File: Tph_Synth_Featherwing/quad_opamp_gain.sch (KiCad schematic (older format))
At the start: 13 parts

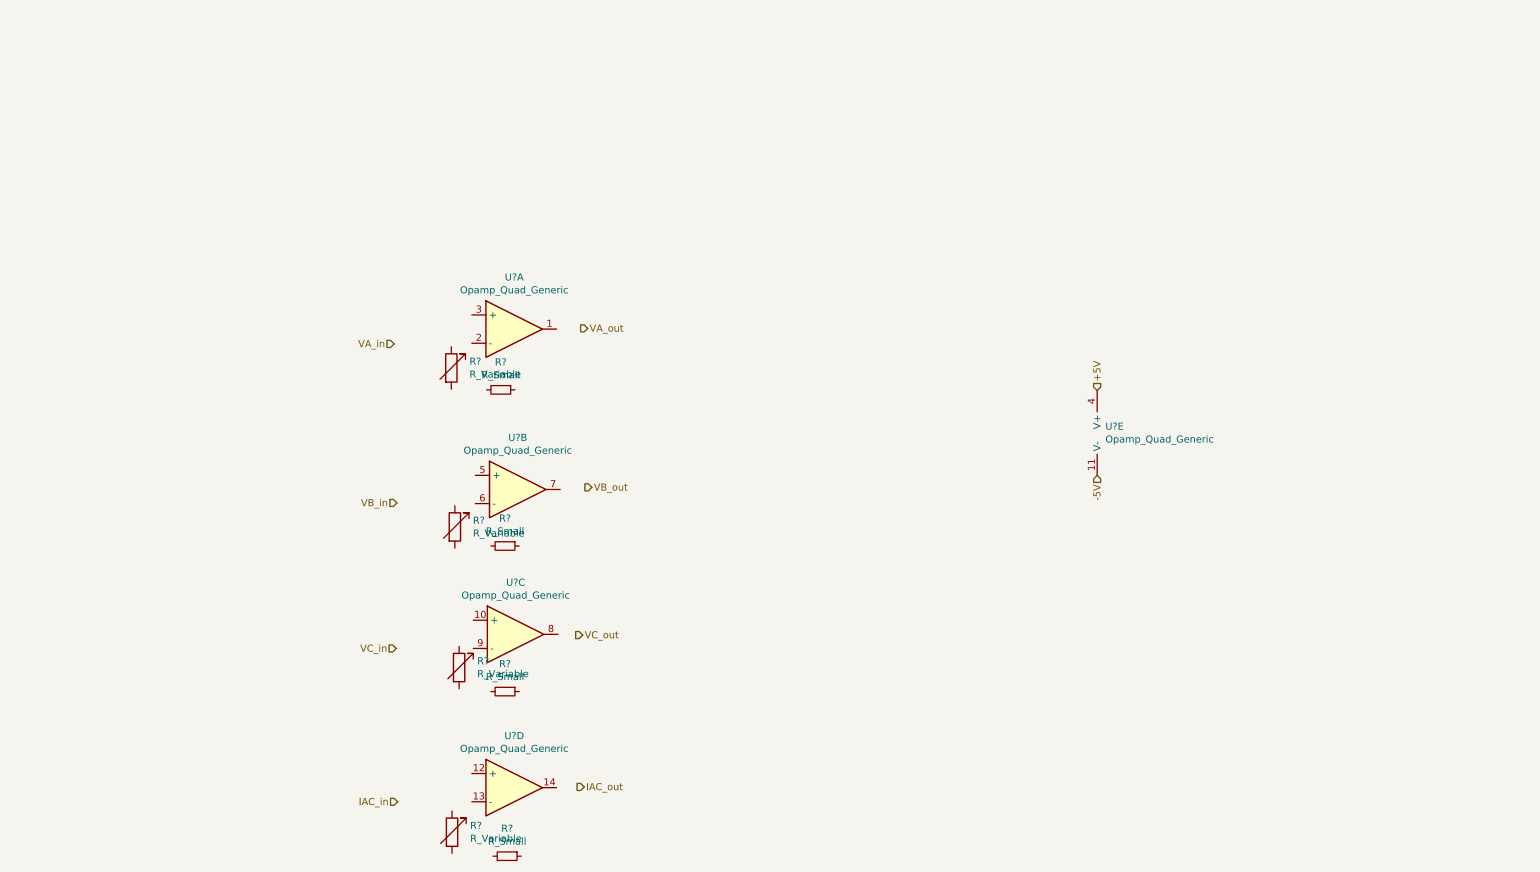
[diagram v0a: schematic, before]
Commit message: Boost-converter and inverting opamps
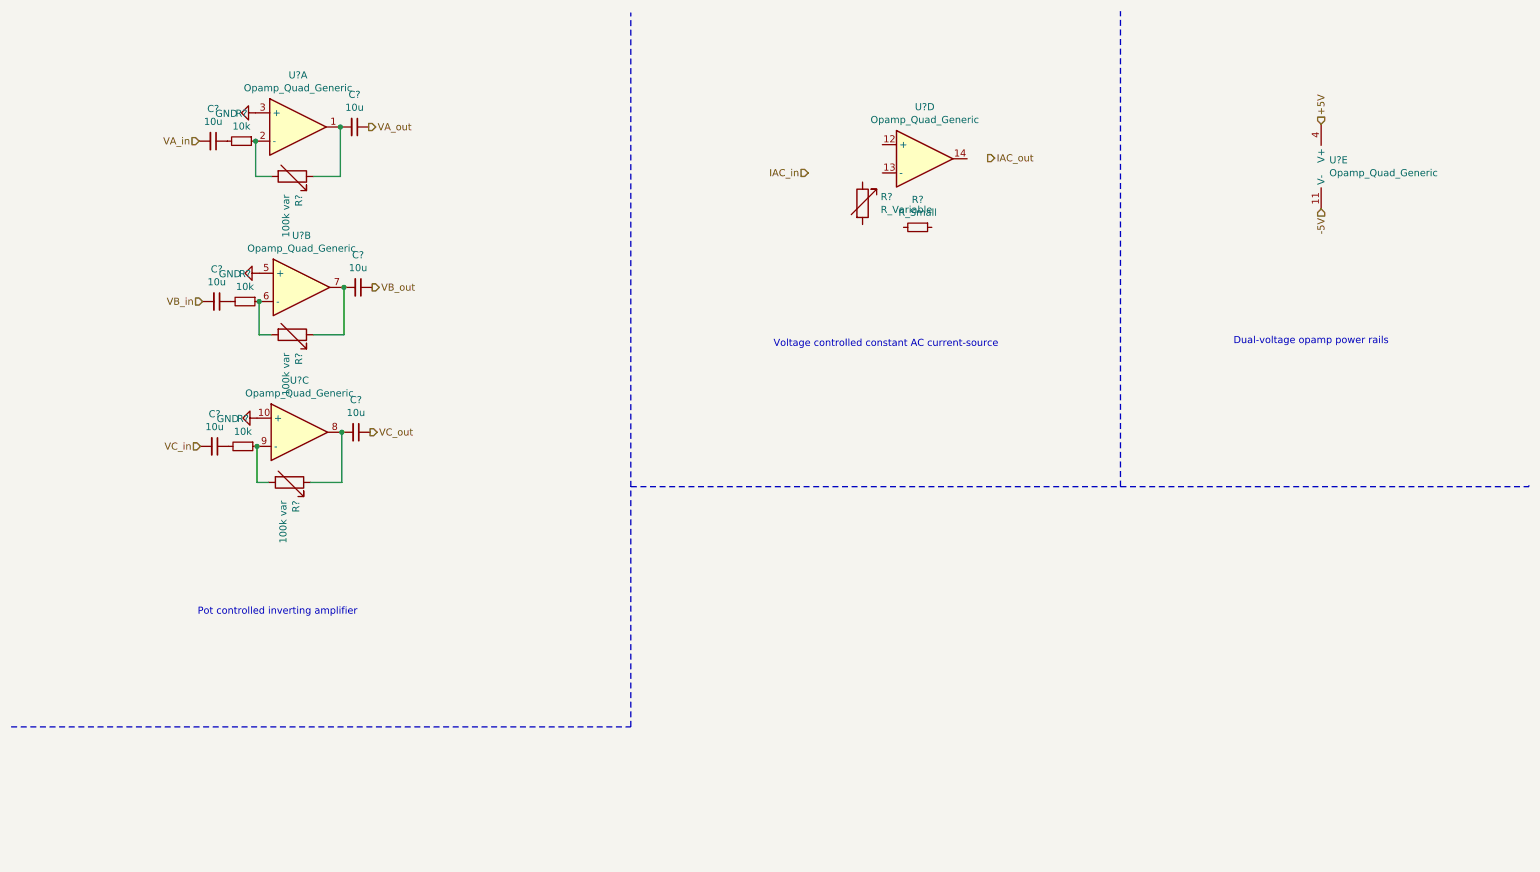
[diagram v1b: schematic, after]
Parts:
- added C? (x6): 10u, symbol Device:C_Small
- R? (x3): value R_Small -> 10k
- R? (x3): value R_Variable -> 100k var
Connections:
- net VA_in: now also C?.2
- net VA_out: now also C?.1
- net VB_in: now also C?.2
- net VB_out: now also C?.1
- net VC_in: now also C?.2
- net VC_out: now also C?.1
- net at U?.1: now also R?.1, C?.2
- net at U?.2 (-): now also R?.1, R?.2
- net GND: now reaches U?.3 (+)
- net GND: now also U?.10 (+), U?.5 (+)
- net at U?.6 (-): now also R?.1, R?.2
- net at U?.7: now also R?.1, C?.2
- net at U?.8: now also R?.1, C?.2
- net at U?.9 (-): now also R?.1, R?.2
- net at R?.2: now also C?.1 (x3)
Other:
- note added: "Dual-voltage opamp power rails"
- note added: "Pot controlled inverting amplifier"
- note added: "Voltage controlled constant AC current-source"
- moved on the sheet: R?, U?A, U?B, U?C, U?D, U?E

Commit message: Added first-cut of schematic
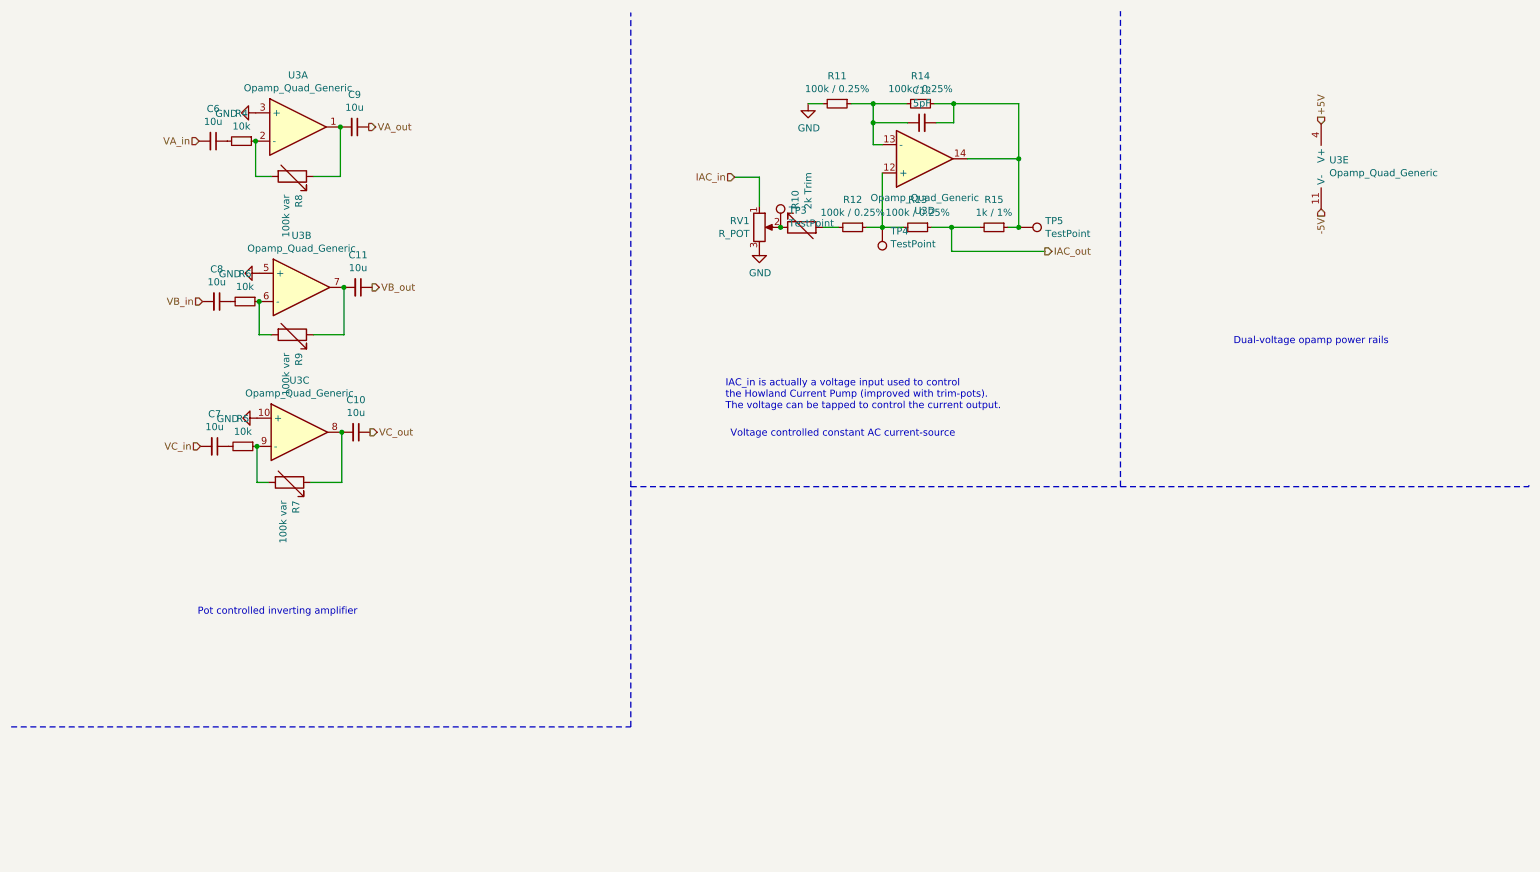
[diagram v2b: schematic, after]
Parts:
- added C12: 5pF, symbol Device:C_Small
- added R11, R12, R14: 100k / 0.25%, symbol Device:R_Small
- added R15: 1k / 1%, symbol Device:R_Small
- added RV1: R_POT, symbol Device:R_POT
- added TP3, TP4, TP5: TestPoint, symbol Connector:TestPoint
- R10: renamed from R?; value R_Variable -> 2k Trim
- R13: renamed from R?; value R_Small -> 100k / 0.25%
- gave numbers to parts that had none: 13
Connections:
- net GND: now also R11.2, RV1.3
- net IAC_in: now also RV1.1
- net IAC_out: now also R13.1, R15.2
- net at U3.12 (+): now also R13.2, R12.1, TP4.1
- net at U3.13 (-): now also C12.1, R11.1, R14.2
- net at U3.14: now also C12.2, R14.1, R15.1, TP5.1
- net at R10.1: now also RV1.2, TP3.1
- net at R10.2: now also R12.2
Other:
- note added: "IAC_in is actually a voltage input used to control\nthe Howland Current Pump (improved with trim-pots).\nThe voltage can be tapped to control the current output."
- moved on the sheet: R10

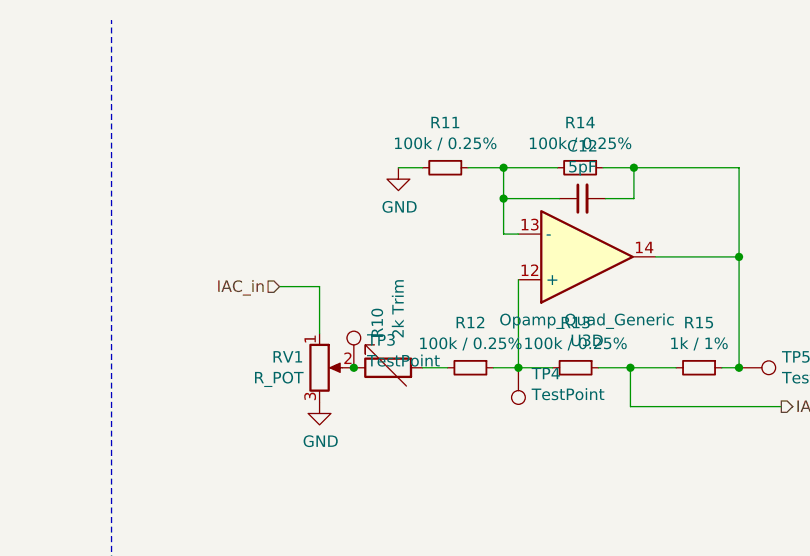
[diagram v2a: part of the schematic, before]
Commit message: Initial attempt at PCB
Signed-off-by: Tisham Dhar <whatnickd@gmail.com>
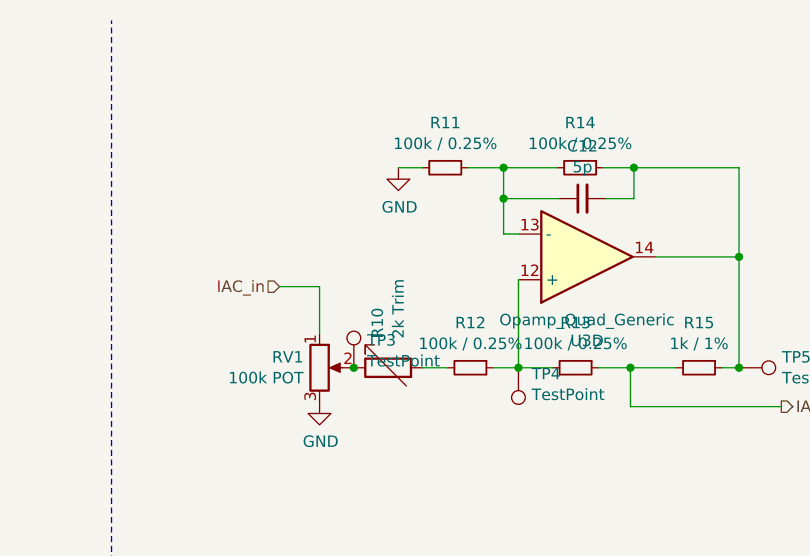
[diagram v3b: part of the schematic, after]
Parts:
- C10, C11, C6, C7, C8, C9: footprint (none) -> Capacitor_SMD:C_0805_2012Metric
- C12: value 5pF -> 5p; footprint (none) -> Capacitor_SMD:C_0603_1608Metric
- R10: footprint (none) -> Potentiometer_THT:Potentiometer_Bourns_3296W_Vertical
- R11, R12, R13, R14, R15, R4, R5, R6: footprint (none) -> Resistor_SMD:R_0603_1608Metric
- R7, R8, R9: footprint (none) -> Potentiometer_THT:Potentiometer_Bourns_PTV09A-2_Single_Horizontal
- RV1: value R_POT -> 100k POT; footprint (none) -> Potentiometer_THT:Potentiometer_Bourns_PTV09A-2_Single_Horizontal
- TP3, TP4, TP5: footprint (none) -> TestPoint:TestPoint_Pad_D1.0mm
- U3: footprint (none) -> Package_SO:TSSOP-14_4.4x5mm_P0.65mm
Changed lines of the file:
@@
 F 0 "U3" H 2495 1662 50  0000 C CNN
 F 1 "Opamp_Quad_Generic" H 2495 1571 50  0000 C CNN
-F 2 "" H 2495 1295 50  0001 C CNN
+F 2 "Package_SO:TSSOP-14_4.4x5mm_P0.65mm" H 2495 1295 50  0001 C CNN
 F 3 "~" H 2495 1295 50  0001 C CNN
 	1    2495 1295
@@
 F 0 "U3" H 2520 2797 50  0000 C CNN
 F 1 "Opamp_Quad_Generic" H 2520 2706 50  0000 C CNN
-F 2 "" H 2520 2430 50  0001 C CNN
+F 2 "Package_SO:TSSOP-14_4.4x5mm_P0.65mm" H 2520 2430 50  0001 C CNN
 F 3 "~" H 2520 2430 50  0001 C CNN
 	2    2520 2430
@@
 F 0 "U3" H 2505 3822 50  0000 C CNN
 F 1 "Opamp_Quad_Generic" H 2505 3731 50  0000 C CNN
-F 2 "" H 2505 3455 50  0001 C CNN
+F 2 "Package_SO:TSSOP-14_4.4x5mm_P0.65mm" H 2505 3455 50  0001 C CNN
 F 3 "~" H 2505 3455 50  0001 C CNN
 	3    2505 3455
@@
 F 0 "U3" H 6930 1887 50  0000 C CNN
 F 1 "Opamp_Quad_Generic" H 6930 1796 50  0000 C CNN
-F 2 "" H 6930 1520 50  0001 C CNN
+F 2 "Package_SO:TSSOP-14_4.4x5mm_P0.65mm" H 6930 1520 50  0001 C CNN
 F 3 "~" H 6930 1520 50  0001 C CNN
 	4    6930 1520
@@
 F 0 "U3" H 9793 1621 50  0000 L CNN
 F 1 "Opamp_Quad_Generic" H 9793 1530 50  0000 L CNN
-F 2 "" H 9835 1575 50  0001 C CNN
+F 2 "Package_SO:TSSOP-14_4.4x5mm_P0.65mm" H 9835 1575 50  0001 C CNN
 F 3 "~" H 9835 1575 50  0001 C CNN
 	5    9835 1575
@@
 F 0 "R4" V 1899 1395 50  0000 C CNN
 F 1 "10k" V 1990 1395 50  0000 C CNN
-F 2 "" H 2095 1395 50  0001 C CNN
+F 2 "Resistor_SMD:R_0603_1608Metric" H 2095 1395 50  0001 C CNN
 F 3 "~" H 2095 1395 50  0001 C CNN
 	1    2095 1395
@@
 F 0 "R6" V 1924 2530 50  0000 C CNN
 F 1 "10k" V 2015 2530 50  0000 C CNN
-F 2 "" H 2120 2530 50  0001 C CNN
+F 2 "Resistor_SMD:R_0603_1608Metric" H 2120 2530 50  0001 C CNN
 F 3 "~" H 2120 2530 50  0001 C CNN
 	1    2120 2530
@@
 F 0 "R5" V 1909 3555 50  0000 C CNN
 F 1 "10k" V 2000 3555 50  0000 C CNN
-F 2 "" H 2105 3555 50  0001 C CNN
+F 2 "Resistor_SMD:R_0603_1608Metric" H 2105 3555 50  0001 C CNN
 F 3 "~" H 2105 3555 50  0001 C CNN
 	1    2105 3555
@@
 F 0 "R13" V 6684 2005 50  0000 C CNN
 F 1 "100k / 0.25%" V 6775 2005 50  0000 C CNN
-F 2 "" H 6880 2005 50  0001 C CNN
+F 2 "Resistor_SMD:R_0603_1608Metric" H 6880 2005 50  0001 C CNN
 F 3 "~" H 6880 2005 50  0001 C CNN
 	1    6880 2005
@@
 F 0 "R8" H 2583 1691 50  0000 L CNN
 F 1 "100k var" H 2583 1600 50  0000 L CNN
-F 2 "" V 2385 1645 50  0001 C CNN
+F 2 "Potentiometer_THT:Potentiometer_Bourns_PTV09A-2_Single_Horizontal" V 2385 1645 50  0001 C CNN
 F 3 "~" H 2455 1645 50  0001 C CNN
 	1    2455 1645
@@
 F 0 "R9" H 2583 2811 50  0000 L CNN
 F 1 "100k var" H 2583 2720 50  0000 L CNN
-F 2 "" V 2385 2765 50  0001 C CNN
+F 2 "Potentiometer_THT:Potentiometer_Bourns_PTV09A-2_Single_Horizontal" V 2385 2765 50  0001 C CNN
 F 3 "~" H 2455 2765 50  0001 C CNN
 	1    2455 2765
@@
 F 0 "R7" H 2563 3856 50  0000 L CNN
 F 1 "100k var" H 2563 3765 50  0000 L CNN
-F 2 "" V 2365 3810 50  0001 C CNN
+F 2 "Potentiometer_THT:Potentiometer_Bourns_PTV09A-2_Single_Horizontal" V 2365 3810 50  0001 C CNN
 F 3 "~" H 2435 3810 50  0001 C CNN
 	1    2435 3810
@@
 F 0 "R10" H 6188 2051 50  0000 L CNN
 F 1 "2k Trim" H 6188 1960 50  0000 L CNN
-F 2 "" V 5990 2005 50  0001 C CNN
+F 2 "Potentiometer_THT:Potentiometer_Bourns_3296W_Vertical" V 5990 2005 50  0001 C CNN
 F 3 "~" H 6060 2005 50  0001 C CNN
 	1    6060 2005
@@
 F 0 "C7" V 1676 3555 50  0000 C CNN
 F 1 "10u" V 1767 3555 50  0000 C CNN
-F 2 "" H 1905 3555 50  0001 C CNN
+F 2 "Capacitor_SMD:C_0805_2012Metric" H 1905 3555 50  0001 C CNN
 F 3 "~" H 1905 3555 50  0001 C CNN
 	1    1905 3555
@@
 F 0 "C8" V 1691 2530 50  0000 C CNN
 F 1 "10u" V 1782 2530 50  0000 C CNN
-F 2 "" H 1920 2530 50  0001 C CNN
+F 2 "Capacitor_SMD:C_0805_2012Metric" H 1920 2530 50  0001 C CNN
 F 3 "~" H 1920 2530 50  0001 C CNN
 	1    1920 2530
@@
 F 0 "C6" V 1666 1395 50  0000 C CNN
 F 1 "10u" V 1757 1395 50  0000 C CNN
-F 2 "" H 1895 1395 50  0001 C CNN
+F 2 "Capacitor_SMD:C_0805_2012Metric" H 1895 1395 50  0001 C CNN
 F 3 "~" H 1895 1395 50  0001 C CNN
 	1    1895 1395
@@
 F 0 "C9" V 2666 1295 50  0000 C CNN
 F 1 "10u" V 2757 1295 50  0000 C CNN
-F 2 "" H 2895 1295 50  0001 C CNN
+F 2 "Capacitor_SMD:C_0805_2012Metric" H 2895 1295 50  0001 C CNN
 F 3 "~" H 2895 1295 50  0001 C CNN
 	1    2895 1295
@@
 F 0 "C11" V 2691 2430 50  0000 C CNN
 F 1 "10u" V 2782 2430 50  0000 C CNN
-F 2 "" H 2920 2430 50  0001 C CNN
+F 2 "Capacitor_SMD:C_0805_2012Metric" H 2920 2430 50  0001 C CNN
 F 3 "~" H 2920 2430 50  0001 C CNN
 	1    2920 2430
@@
 F 0 "C10" V 2676 3455 50  0000 C CNN
 F 1 "10u" V 2767 3455 50  0000 C CNN
-F 2 "" H 2905 3455 50  0001 C CNN
+F 2 "Capacitor_SMD:C_0805_2012Metric" H 2905 3455 50  0001 C CNN
 F 3 "~" H 2905 3455 50  0001 C CNN
 	1    2905 3455
@@
 Data
 89 50 4E 47 0D 0A 1A 0A 00 00 00 0D 49 48 44 52 00 00 03 DD 00 00 02 B4 08 02 00 00 00 91 20 C9
-F7 00 00 00 03 73 42 49 54 08 08 08 DB E1 4F E0 00 00 00 09 70 48 59 73 00 00 12 74 00 00 12 74
-01 DE 66 1F 78 00 00 20 00 49 44 41 54 78 9C EC 9D 75 9C 5D C5 F9 FF 3F 33 73 F4 EA BA C5 DD 95
+F7 00 00 00 03 73 42 49 54 08 08 08 DB E1 4F E0 00 00 00 09 70 48 59 73 00 00 12 5C 00 00 12 5C
+01 68 C4 36 89 00 00 20 00 49 44 41 54 78 9C EC 9D 75 9C 5D C5 F9 FF 3F 33 73 F4 EA BA C5 DD 95
 18 21 21 48 08 04 29 52 08 1E 82 53 28 05 0A 7C 69 A1 48 03 85 D2 E2 1E DC 2D 85 62 49 71 02 09
 14 27 01 02 81 00 21 AE 2B D7 8F 8C FC FE 38 BB CB 12 52 81 B6 24 FD 75 DE AF 7D ED DE BD 72 CE
@@
 F 0 "R14" V 6704 1130 50  0000 C CNN
 F 1 "100k / 0.25%" V 6795 1130 50  0000 C CNN
-F 2 "" H 6900 1130 50  0001 C CNN
+F 2 "Resistor_SMD:R_0603_1608Metric" H 6900 1130 50  0001 C CNN
 F 3 "~" H 6900 1130 50  0001 C CNN
 	1    6900 1130
@@
 F 0 "R11" V 6114 1130 50  0000 C CNN
 F 1 "100k / 0.25%" V 6205 1130 50  0000 C CNN
-F 2 "" H 6310 1130 50  0001 C CNN
+F 2 "Resistor_SMD:R_0603_1608Metric" H 6310 1130 50  0001 C CNN
 F 3 "~" H 6310 1130 50  0001 C CNN
 	1    6310 1130
@@
 P 6910 1265
 F 0 "C12" V 7139 1265 50  0000 C CNN
-F 1 "5pF" V 7048 1265 50  0000 C CNN
-F 2 "" H 6910 1265 50  0001 C CNN
+F 1 "5p" V 7048 1265 50  0000 C CNN
+F 2 "Capacitor_SMD:C_0603_1608Metric" H 6910 1265 50  0001 C CNN
 F 3 "~" H 6910 1265 50  0001 C CNN
 	1    6910 1265
@@
 F 0 "R15" V 7224 2005 50  0000 C CNN
 F 1 "1k / 1%" V 7315 2005 50  0000 C CNN
-F 2 "" H 7420 2005 50  0001 C CNN
+F 2 "Resistor_SMD:R_0603_1608Metric" H 7420 2005 50  0001 C CNN
 F 3 "~" H 7420 2005 50  0001 C CNN
 	1    7420 2005
@@
 F 0 "R12" V 6224 2005 50  0000 C CNN
 F 1 "100k / 0.25%" V 6315 2005 50  0000 C CNN
-F 2 "" H 6420 2005 50  0001 C CNN
+F 2 "Resistor_SMD:R_0603_1608Metric" H 6420 2005 50  0001 C CNN
 F 3 "~" H 6420 2005 50  0001 C CNN
 	1    6420 2005
@@
 P 5760 2005
 F 0 "RV1" H 5690 2051 50  0000 R CNN
-F 1 "R_POT" H 5690 1960 50  0000 R CNN
-F 2 "" H 5760 2005 50  0001 C CNN
+F 1 "100k POT" H 5690 1960 50  0000 R CNN
+F 2 "Potentiometer_THT:Potentiometer_Bourns_PTV09A-2_Single_Horizontal" H 5760 2005 50  0001 C CNN
 F 3 "~" H 5760 2005 50  0001 C CNN
 	1    5760 2005
@@
 F 0 "TP4" H 6572 2032 50  0000 R CNN
 F 1 "TestPoint" H 6572 2123 50  0000 R CNN
-F 2 "" H 6830 2005 50  0001 C CNN
+F 2 "TestPoint:TestPoint_Pad_D1.0mm" H 6830 2005 50  0001 C CNN
 F 3 "~" H 6830 2005 50  0001 C CNN
 	1    6630 2005
@@
 F 0 "TP5" V 7549 2193 50  0000 L CNN
 F 1 "TestPoint" V 7640 2193 50  0000 L CNN
-F 2 "" H 7795 2005 50  0001 C CNN
+F 2 "TestPoint:TestPoint_Pad_D1.0mm" H 7795 2005 50  0001 C CNN
 F 3 "~" H 7795 2005 50  0001 C CNN
 	1    7595 2005
@@
 F 0 "TP3" H 5968 2125 50  0000 L CNN
 F 1 "TestPoint" H 5968 2034 50  0000 L CNN
-F 2 "" H 6110 2005 50  0001 C CNN
+F 2 "TestPoint:TestPoint_Pad_D1.0mm" H 6110 2005 50  0001 C CNN
 F 3 "~" H 6110 2005 50  0001 C CNN
 	1    5910 2005
